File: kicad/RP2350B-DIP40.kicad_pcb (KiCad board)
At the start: 2 copper layers, 54 x 21.6 mm, 30 parts, among them J1 USB_C_Receptacle_USB2.0_16P, J2 Conn_ARM_JTAG_SWD_10, J3 Conn_01x03_Socket, J4 qwiic, J5 Micro_SD_Card, U1 TPD2EUSB30, U2 Picossci_B2_RB2350B, U3 18F47Q43, U4 TPS22917DBV

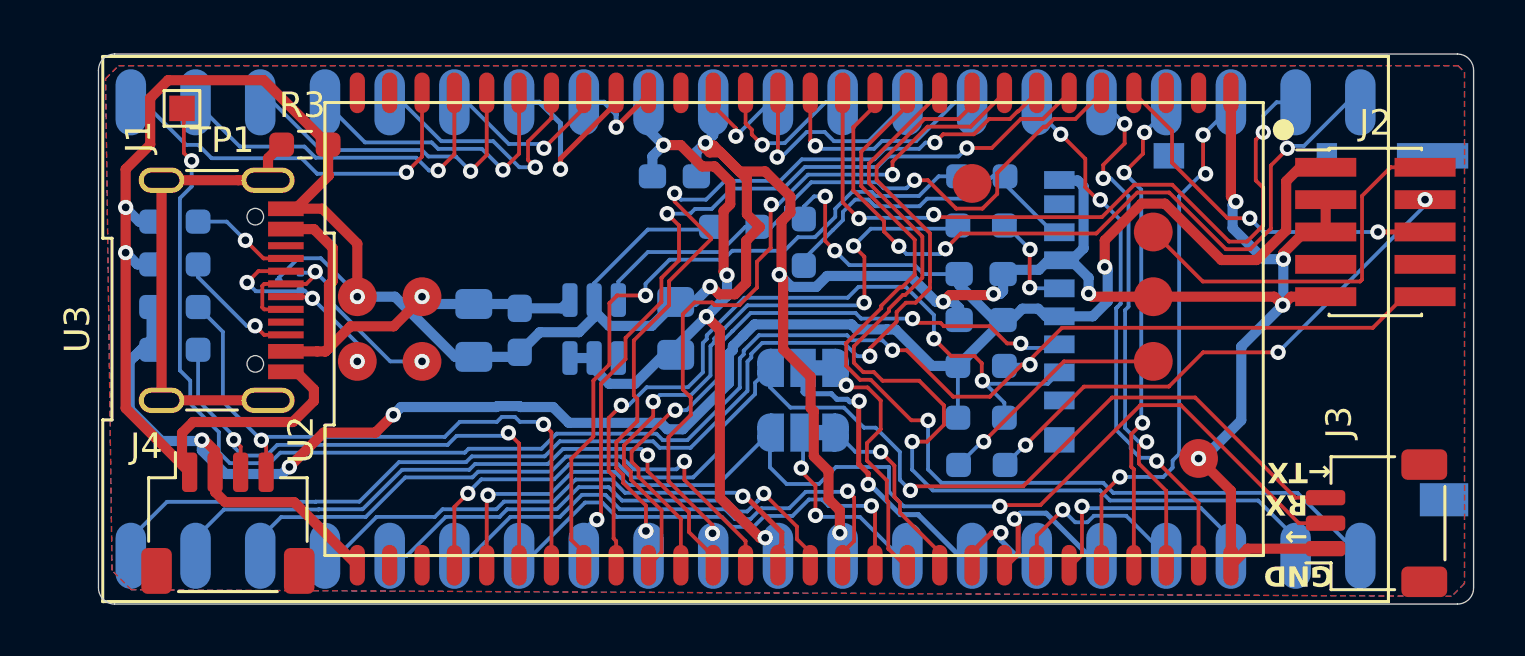
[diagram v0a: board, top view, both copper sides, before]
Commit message: Add PCB design RP2350B-DIP40-rev1.0
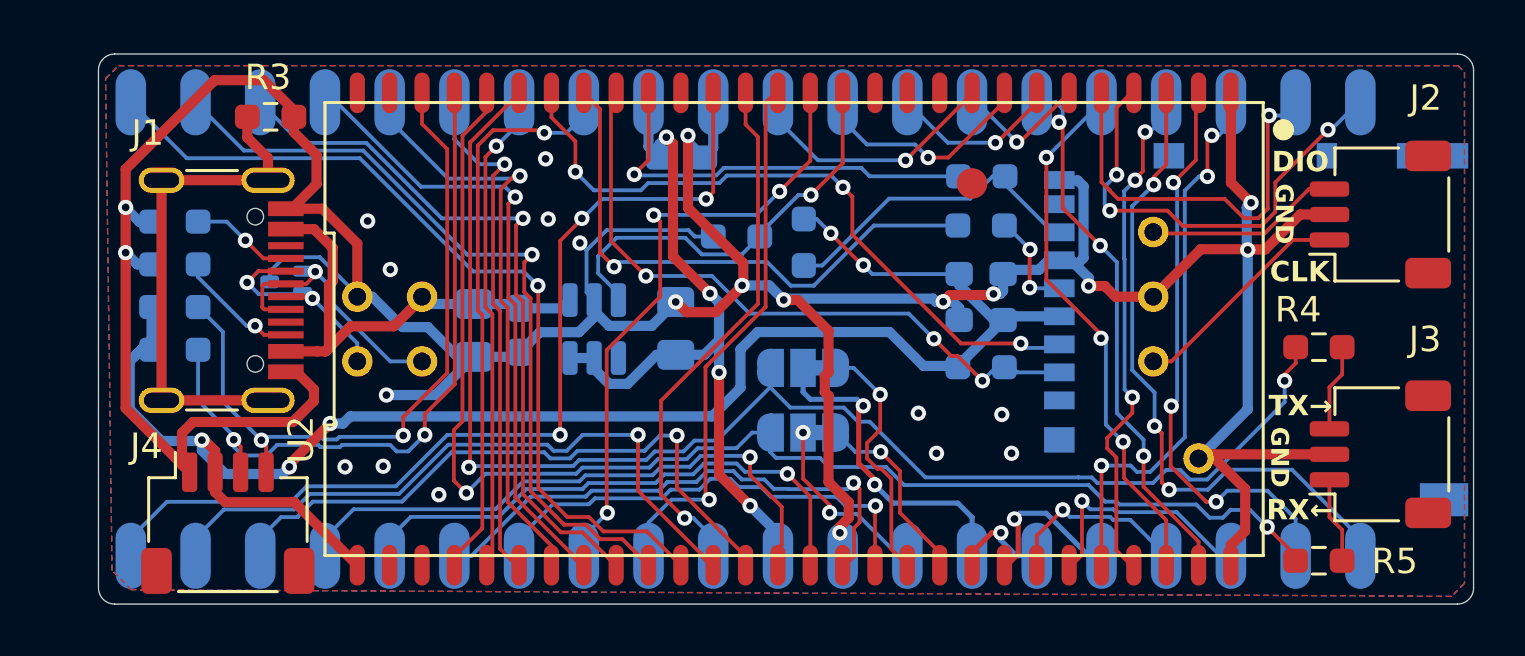
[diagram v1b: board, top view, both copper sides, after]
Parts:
- removed TP1: TestPoint, TestPoint:TestPoint_Pad_1.0x1.0mm
- J2: value Conn_ARM_JTAG_SWD_10 -> debug connector; footprint Connector_PinHeader_1.27mm:PinHeader_2x05_P1.27mm_Vertical_SMD -> Connector_JST:JST_SH_SM03B-SRSS-TB_1x03-1MP_P1.00mm_Horizontal
- J3: value Conn_01x03_Socket -> uart connector
- R4: value 10K -> 33R; moved to F.Cu
- R5: moved to F.Cu
- moved R5 13.8 mm to (153.6, 131.3), turned to 180 degrees
- moved R4 13.3 mm to (153.6, 122.9), turned to 180 degrees
- moved J3 2.71 mm to (156.0, 127.1)
- moved R9 1.98 mm to (140.3, 123.7)
- moved R3 1.73 mm to (112.4, 113.9)
- moved C4 0.79 mm to (128.5, 115.5)
- moved J2 0.71 mm to (156.0, 117.7), turned to 90 degrees
- moved R8 0.39 mm to (130.7, 118.6)
- moved U1 0.13 mm to (113.0, 120.4)
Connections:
- J2 pad 1: +3.3V -> SWCLK
- J2 pad 2: SWDIO -> GND
- J2 pad 3: GND -> SWDIO
- J3 pad 1: GND -> Net-(J3-RX)
- J3 pad 2: UART0_RX -> GND
- J3 pad 3: UART0_TX -> Net-(J3-TX)
- R4 pad 1: +3.3V -> Net-(J3-TX)
- R4 pad 2: nRESET -> UART0_TX
- R5 pad 1: SWCLK -> Net-(J3-RX)
- R5 pad 2: Net-(J2-SWCLK/TCK) -> UART0_RX
- U2 pad 10: SCK -> RB6
- U2 pad 11: MOSI -> RB7
- U2 pad 30: unconnected-(U2-GP24(LED1)-Pad30) -> RD0
- U2 pad 31: unconnected-(U2-GP25(LED2)-Pad31) -> RD1
- U2 pad 32: SWO -> RD2
- U2 pad 33: 5V_OUT_EN -> RD3
- U2 pad 34: RE0 -> RD4
- U2 pad 35: RE1 -> RD5
- U2 pad 36: RE2 -> RD6
- U2 pad 37: RE3 -> RD7
- U2 pad 38: RD0 -> unconnected-(U2-GP32-Pad38)
- U2 pad 39: RD1 -> unconnected-(U2-GP33-Pad39)
- U2 pad 4: UART0_TX -> RB0
- U2 pad 40: RD2 -> unconnected-(U2-GP34-Pad40)
- U2 pad 41: RD3 -> 5V_OUT_EN
- U2 pad 42: RD4 -> RE0
- U2 pad 43: RD5 -> RE1
- U2 pad 44: RD6 -> RE2
- U2 pad 45: RD7 -> RE3
- U2 pad 47: RB0 -> MISO
- U2 pad 48: RB1 -> SPI_CS
- U2 pad 49: RB2 -> SCK
- U2 pad 5: UART0_RX -> RB1
- U2 pad 50: RB3 -> MOSI
- U2 pad 51: RB4 -> UART0_TX
- U2 pad 52: RB5 -> UART0_RX
- U2 pad 53: RB6 -> SDA
- U2 pad 54: RB7 -> SCL
- U2 pad 6: SDA -> RB2
- U2 pad 7: SCL -> RB3
- U2 pad 8: MISO -> RB4
- U2 pad 9: SPI_CS -> RB5
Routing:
- net nRESET: track 68.8 -> 0.00 mm, vias 3 -> 0
- net +3.3V: track 88.7 -> 66.2 mm, vias 6 -> 5
- net Net-(J2-SWCLK/TCK): track 20.9 -> 0.00 mm, vias 3 -> 0
- net RB0: track 3.84 -> 22.3 mm
- net RB7: track 15.4 -> 33.8 mm
- net RB6: track 13.9 -> 31.0 mm
- net RB5: track 12.7 -> 28.1 mm
- net RD0: track 38.3 -> 23.1 mm, vias 1 -> 3
- net RB4: track 11.4 -> 26.0 mm
- net SWO: track 14.4 -> 0.00 mm, vias 2 -> 0
- net RD3: track 28.9 -> 15.7 mm, vias 3 -> 1
- net RB3: track 10.2 -> 23.4 mm
- net RB2: track 7.08 -> 20.2 mm
- net RD2: track 31.1 -> 18.0 mm
- net RE1: track 33.1 -> 21.3 mm, vias 3 -> 1
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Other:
- board text added: "@hanyazou Mar 22, 2026"
- board text added: "CLK"
- board text added: "DIO"
- board text added: "RP2350B-DIP40 rev 1.0"
- board text added: "RX←"
- board text added: "TX→"
- board text removed: "RP2350B-DIP40 rev 0.8 @hanyazou Mar 7, 2026"
- board text removed: "←TX"
- board text removed: "→ RX"
